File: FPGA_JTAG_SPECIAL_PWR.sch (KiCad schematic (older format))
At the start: 31 parts, among them J2 Reset_Switch, U900 GW1N-9LQ100

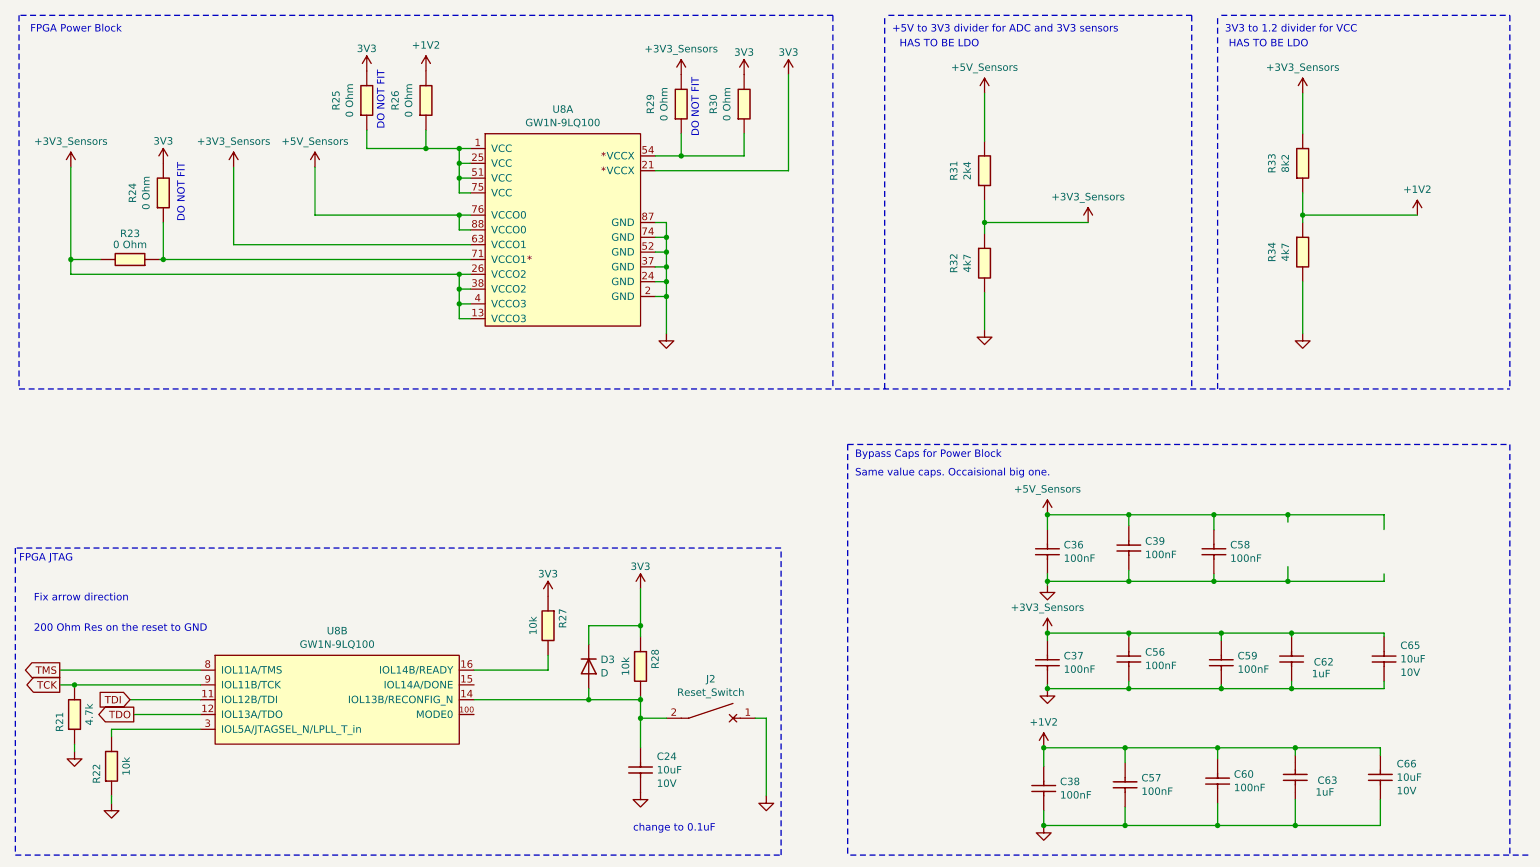
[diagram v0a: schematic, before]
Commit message: First cut at a 3D rendering of the board.  Not too many missing models...
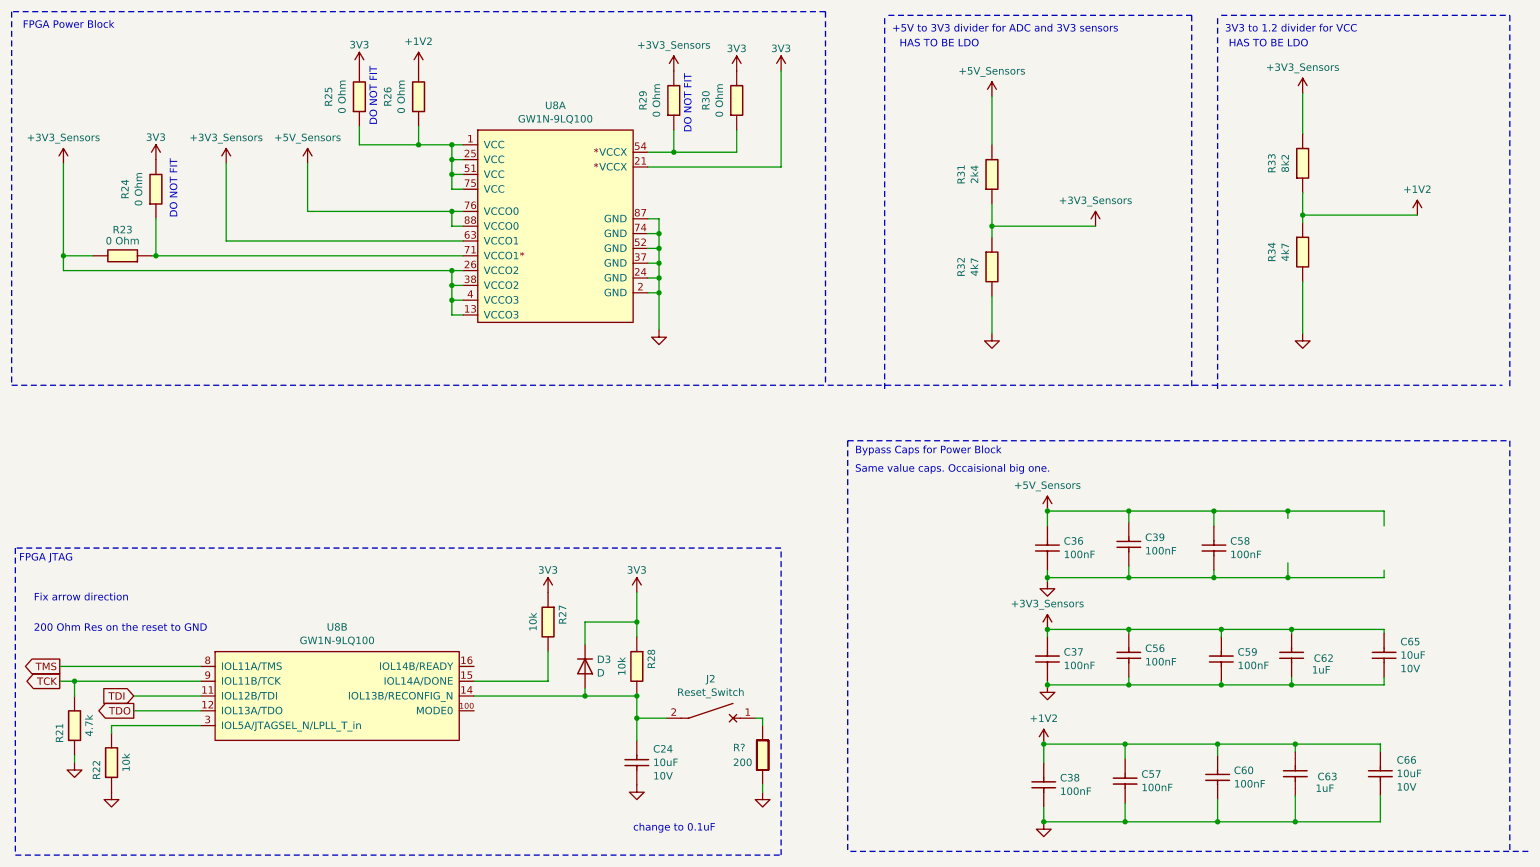
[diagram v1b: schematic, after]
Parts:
- added R?: R_0603_200_0.1W_1%, Resistor_SMD:R_0603_1608Metric, symbol OpenVent:R_0603_200_0.1W_1%
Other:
- moved on the sheet: C24, C36, C37, C38, C39, C56, C57, C58, C59, C60, C62, C63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
